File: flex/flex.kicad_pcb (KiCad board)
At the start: 2 copper layers, 74.1 x 41.5 mm, 33 parts, among them J1 Conn_01x06_Female, J2 Conn_01x03_Female, J3 Conn_01x01_Female, SW1 SW_Push, SW14 SW_Push, SW19 SW_Push, SW5 SW_Push, SW9 SW_Push

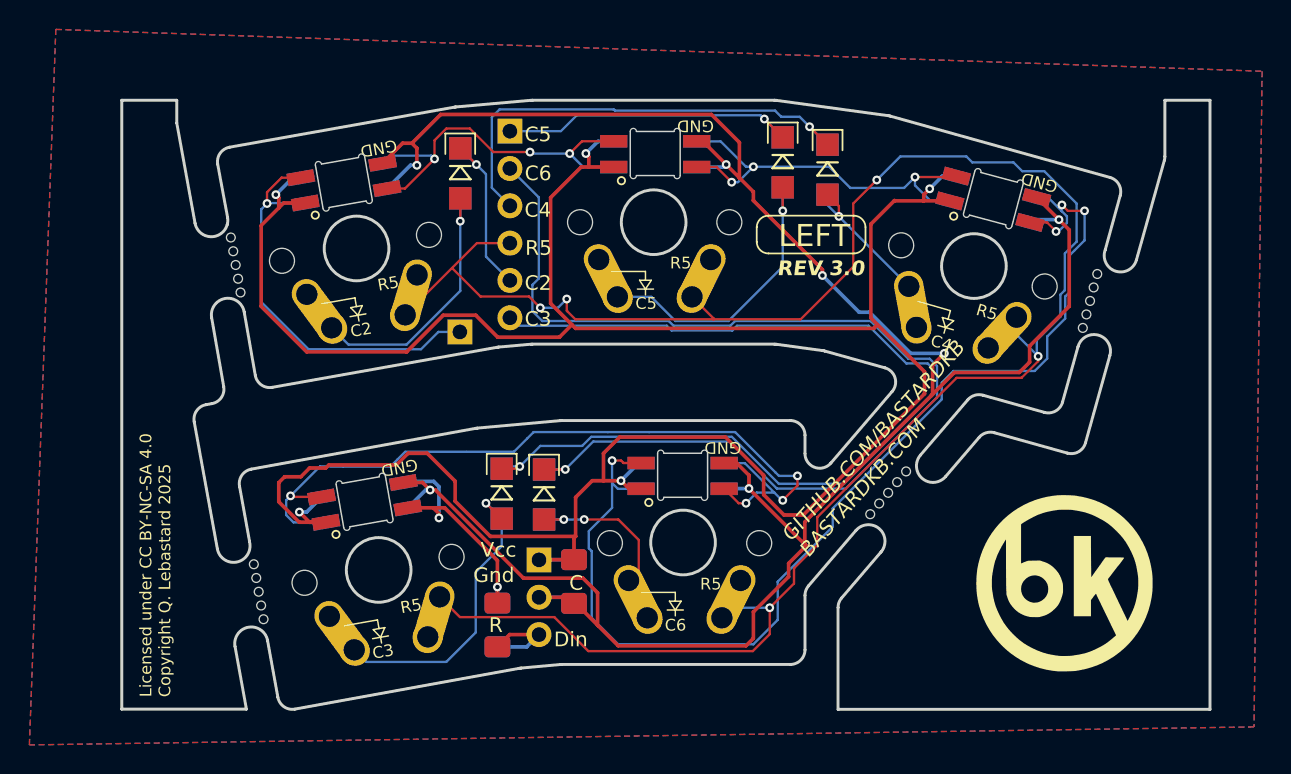
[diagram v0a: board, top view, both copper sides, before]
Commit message: edge cuts
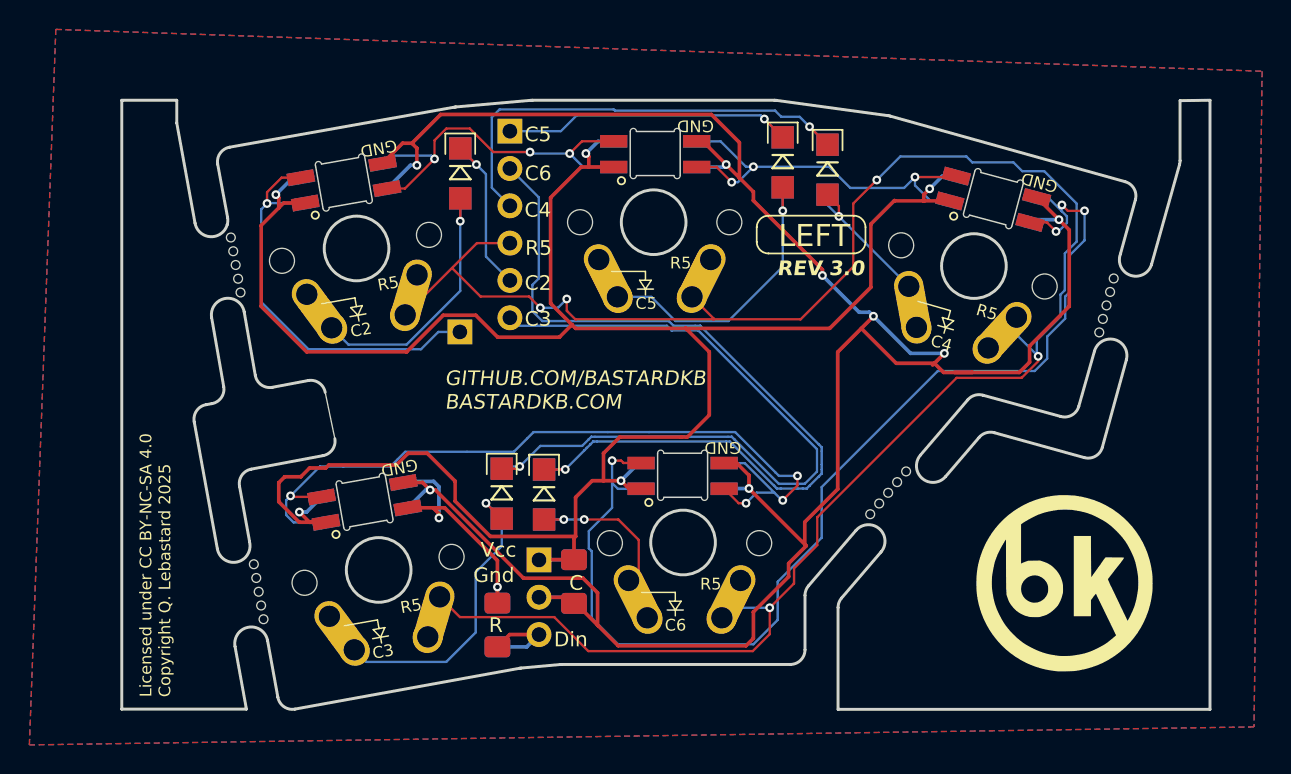
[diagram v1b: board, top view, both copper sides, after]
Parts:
- moved Mousebite2 1.16 mm to (125.0, 80.2)
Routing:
- net Vcc: track 177.6 -> 155.6 mm
- net col3: track 67.7 -> 51.5 mm
- net col6: track 75.1 -> 58.9 mm
- net Gnd: track 155.9 -> 164.1 mm, vias 7 -> 8
- net Net-(D4-DOUT): track 77.6 -> 78.2 mm
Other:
- outline, holes or cut-outs redrawn
